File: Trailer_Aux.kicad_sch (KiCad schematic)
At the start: 19 parts, among them Q44 IRF4905PBF, Q68 2N7000, SW11 KSD9700, SW7 SW_SPST, U12 LM339

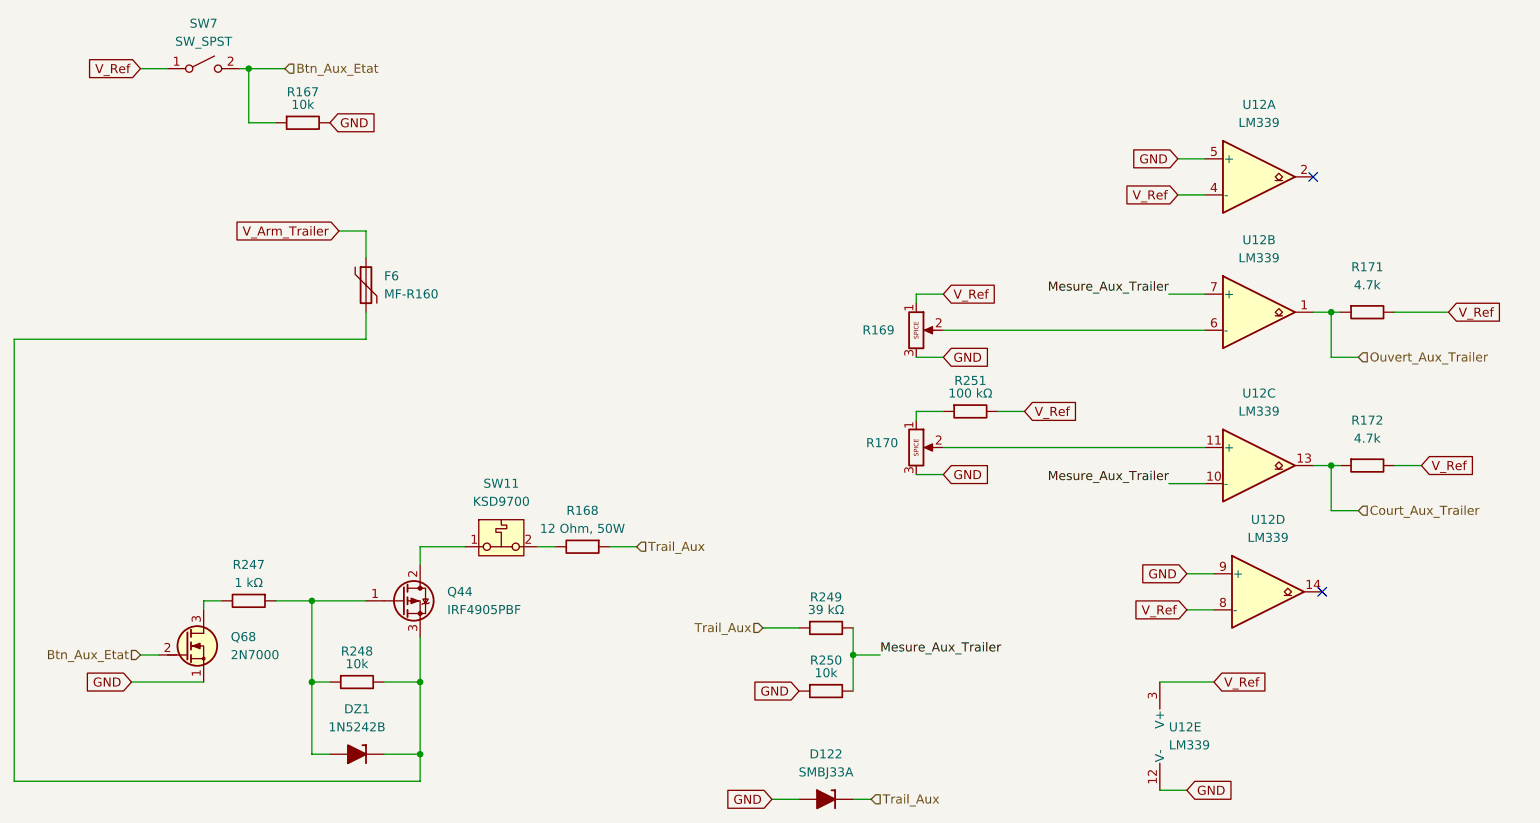
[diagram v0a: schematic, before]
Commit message: Add files via upload
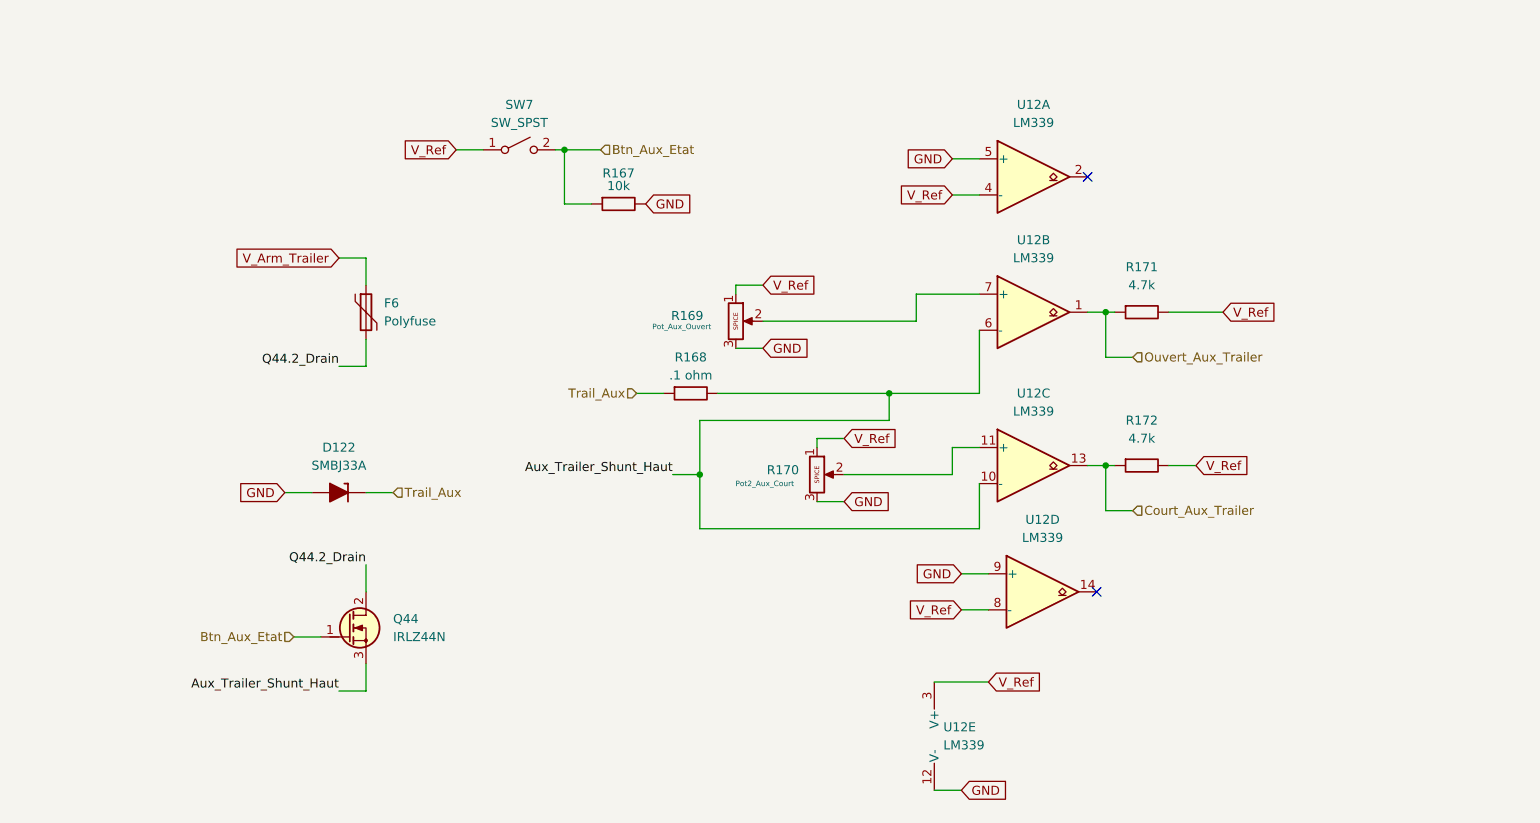
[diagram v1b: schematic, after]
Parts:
- removed DZ1: 1N5242B, PCM_Diode_THT_AKL:D_DO-35_SOD27_P7.62mm_Horizontal_Zener, symbol PCM_Diode_Zener_AKL:1N5242B
- removed Q68: 2N7000, PCM_Package_TO_SOT_THT_AKL:TO-92_Inline_Wide_SGD, symbol PCM_Transistor_MOSFET_AKL:2N7000
- removed R247: 1 kΩ, Resistor_THT:R_Axial_DIN0207_L6.3mm_D2.5mm_P10.16mm_Horizontal, symbol PCM_SL_Resistors:4.7k
- removed R248, R250: 10k, Resistor_THT:R_Axial_DIN0207_L6.3mm_D2.5mm_P10.16mm_Horizontal, symbol PCM_SL_Resistors:10k
- removed R249: 39 kΩ, Resistor_THT:R_Axial_DIN0207_L6.3mm_D2.5mm_P10.16mm_Horizontal, symbol PCM_SL_Resistors:10k
- removed R251: 100 kΩ, Resistor_THT:R_Axial_DIN0207_L6.3mm_D2.5mm_P10.16mm_Horizontal, symbol PCM_SL_Resistors:10k
- removed SW11: KSD9700, symbol Switch:SW_SPST_Temperature_NC
- F6: value MF-R160 -> Polyfuse
- Q44: value IRF4905PBF -> IRLZ44N; footprint Package_TO_SOT_THT:TO-220-3_Vertical -> PCM_Package_TO_SOT_THT_AKL:TO-220-3_Vertical_GDS; symbol Transistor_FET:IRF4905 -> PCM_Transistor_MOSFET_AKL:IRLZ44N
- R168: value 12 Ohm, 50W -> .1 ohm; footprint TerminalBlock_Phoenix:TerminalBlock_Phoenix_PT-1,5-2-3.5-H_1x02_P3.50mm_Horizontal -> Resistor_THT:R_Axial_DIN0207_L6.3mm_D2.5mm_P10.16mm_Horizontal
- R169, R170: footprint TRIM_3296W1103LF:TRIM_3296W1103LF -> (none)
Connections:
- net Btn_Aux_Etat: now also Q44.1 (G)
- net V_Ref: now also R170.1
- net Q44.2_Drain: now reaches Q44.2 (D)
- net Q44.2_Drain: now also F6.2
- net Aux_Trailer_Shunt_Haut: now reaches Q44.3 (S)
- net Aux_Trailer_Shunt_Haut: now also R168.2, U12.10 (-), U12.6 (-); no longer F6.2
- net at R169.2: now also U12.7 (+); no longer U12.6 (-)
- removed net Mesure_Aux_Trailer: U12.10 (-), U12.7 (+)
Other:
- moved on the sheet: D122, F6, R167, R168, R169, R171, R172, SW7, U12A, U12B, U12C, U12D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

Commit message: Add files via upload
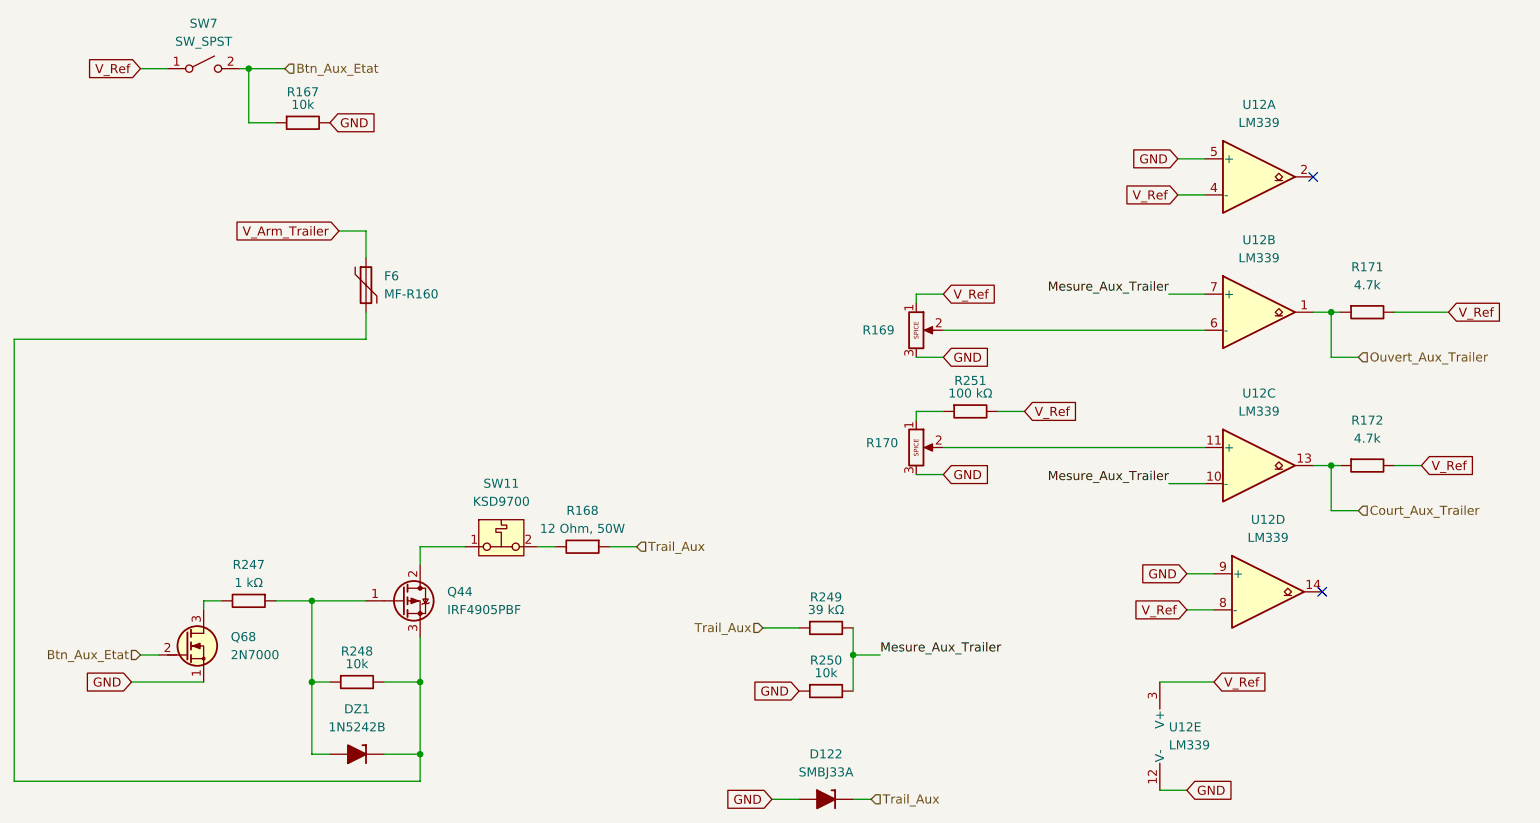
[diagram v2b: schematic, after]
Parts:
- added DZ1: 1N5242B, PCM_Diode_THT_AKL:D_DO-35_SOD27_P7.62mm_Horizontal_Zener, symbol PCM_Diode_Zener_AKL:1N5242B
- added Q68: 2N7000, PCM_Package_TO_SOT_THT_AKL:TO-92_Inline_Wide_SGD, symbol PCM_Transistor_MOSFET_AKL:2N7000
- added R247: 1 kΩ, Resistor_THT:R_Axial_DIN0207_L6.3mm_D2.5mm_P10.16mm_Horizontal, symbol PCM_SL_Resistors:4.7k
- added R248, R250: 10k, Resistor_THT:R_Axial_DIN0207_L6.3mm_D2.5mm_P10.16mm_Horizontal, symbol PCM_SL_Resistors:10k
- added R249: 39 kΩ, Resistor_THT:R_Axial_DIN0207_L6.3mm_D2.5mm_P10.16mm_Horizontal, symbol PCM_SL_Resistors:10k
- added R251: 100 kΩ, Resistor_THT:R_Axial_DIN0207_L6.3mm_D2.5mm_P10.16mm_Horizontal, symbol PCM_SL_Resistors:10k
- added SW11: KSD9700, symbol Switch:SW_SPST_Temperature_NC
- F6: value Polyfuse -> MF-R160
- Q44: value IRLZ44N -> IRF4905PBF; footprint PCM_Package_TO_SOT_THT_AKL:TO-220-3_Vertical_GDS -> Package_TO_SOT_THT:TO-220-3_Vertical; symbol PCM_Transistor_MOSFET_AKL:IRLZ44N -> Transistor_FET:IRF4905
- R168: value .1 ohm -> 12 Ohm, 50W; footprint Resistor_THT:R_Axial_DIN0207_L6.3mm_D2.5mm_P10.16mm_Horizontal -> TerminalBlock_Phoenix:TerminalBlock_Phoenix_PT-1,5-2-3.5-H_1x02_P3.50mm_Horizontal
- R169, R170: footprint (none) -> TRIM_3296W1103LF:TRIM_3296W1103LF
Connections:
- net Btn_Aux_Etat: now also Q68.2 (G); no longer Q44.1 (G)
- net GND: now also Q68.1 (S), R250.1
- net Trail_Aux: now also R249.1
- net V_Ref: now also R251.2; no longer R170.1
- net at R169.2: now also U12.6 (-); no longer U12.7 (+)
- removed net Aux_Trailer_Shunt_Haut: Q44.3 (S), R168.2, U12.10 (-), U12.6 (-)
- net Q44.2_Drain: no longer names the net of Q44.2 (D)
- net Q44.2_Drain: now also SW11.1; no longer F6.2
- new net: Q68.3 (D), R247.2
- new net: DZ1.2 (A), Q44.1 (G), R247.1, R248.1
- new net: DZ1.1 (K), F6.2, Q44.3 (S), R248.2
- new net: R168.2, SW11.2
- new net: R170.1, R251.1
- new net Mesure_Aux_Trailer: R249.2, R250.2, U12.10 (-), U12.7 (+)
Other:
- moved on the sheet: D122, F6, R167, R168, R169, R171, R172, SW7, U12A, U12B, U12C, U12D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
